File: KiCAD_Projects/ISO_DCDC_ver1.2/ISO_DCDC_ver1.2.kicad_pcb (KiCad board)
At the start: 2 copper layers, 60 x 60 mm, 51 parts, among them IC4 PC817, IC5 PC817, P1 CONN_01X01, P10 CONN_01X02, P12 CONN_01X01, P13 CONN_01X04, P14 CONN_01X02, P2 CONN_01X01, P21 CONN_01X02, P22 CONN_01X01, P23 CONN_01X01, P25 CONN_01X01, P26 CONN_01X01, P3 CONN_01X01, P4 CONN_01X02, P5 CONN_01X02, P6 CONN_01X02, P7 CONN_01X02, P8 CONN_01X01, Q1 MOSFET_N, U1 V23076-D3001-D142, U3 V23076-D3001-D142

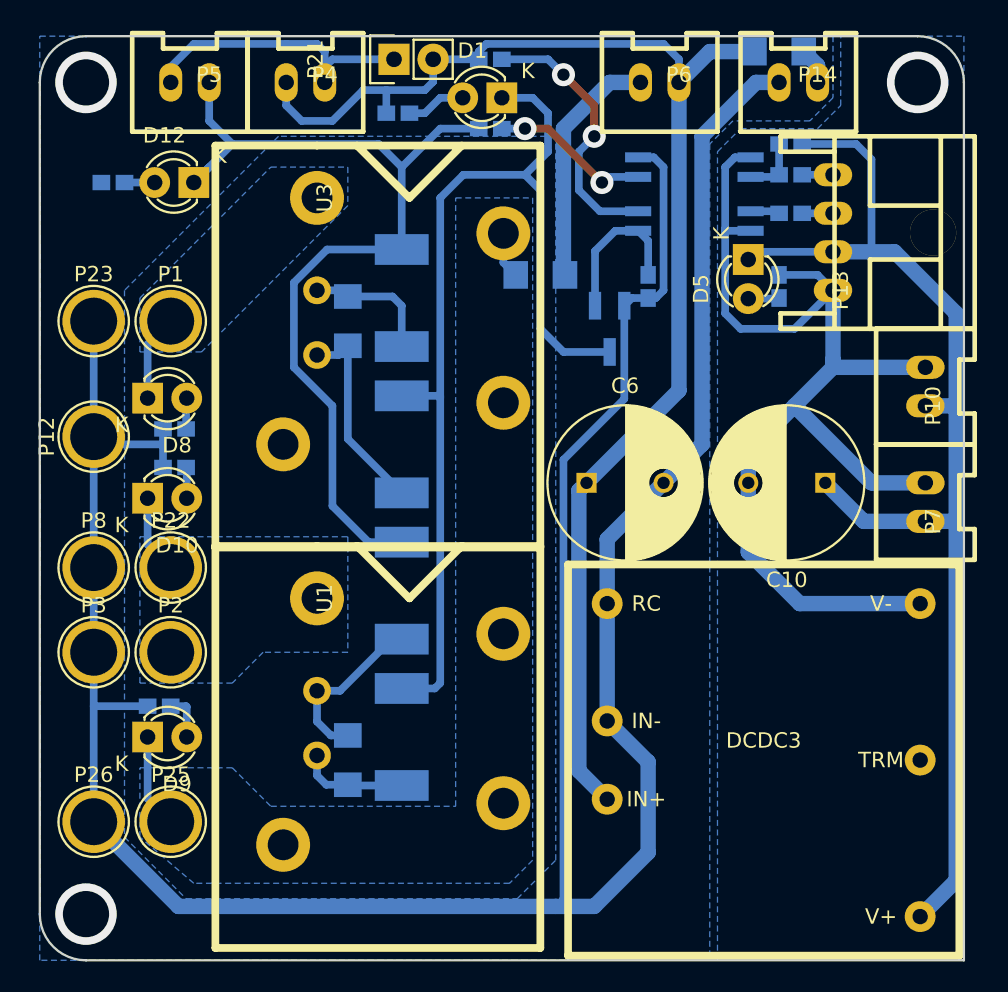
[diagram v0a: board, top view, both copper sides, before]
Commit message: 電源基板ver1.2加工した｡次ver1.3作るべきかも
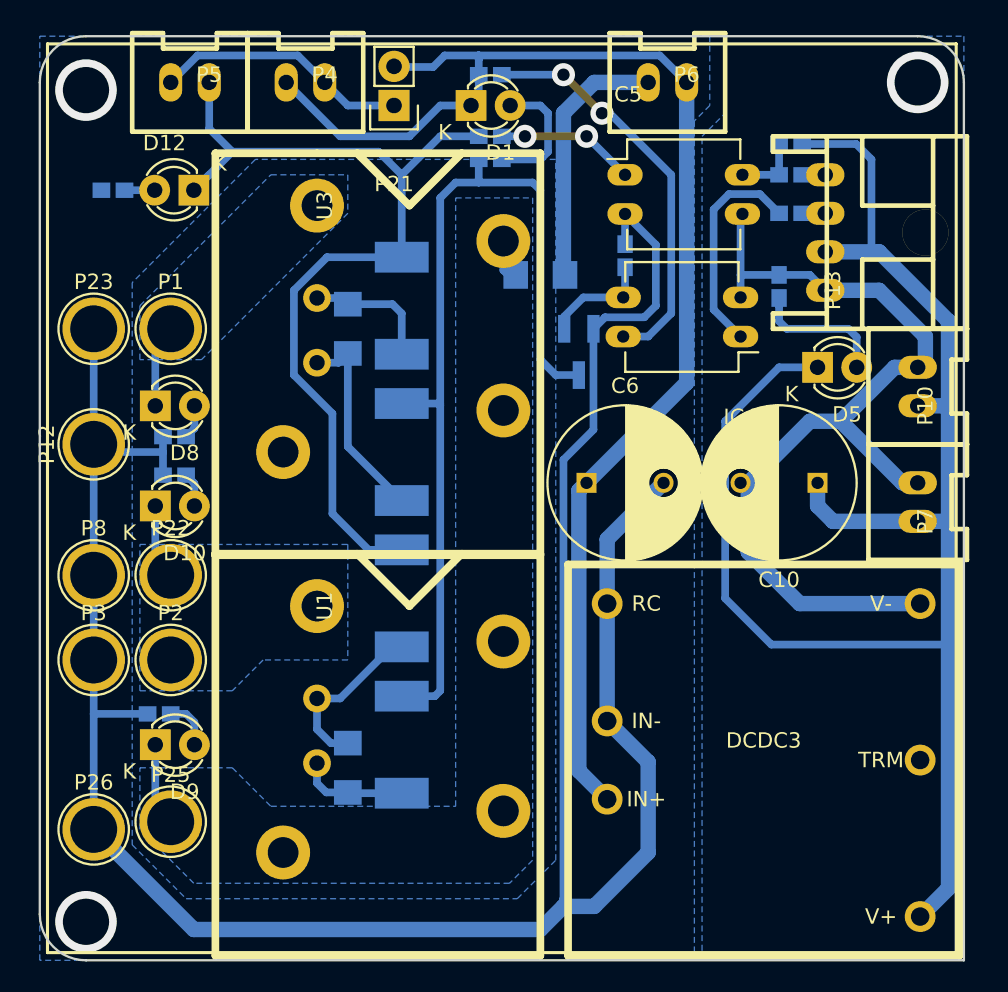
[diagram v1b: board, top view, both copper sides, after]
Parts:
- removed D4: DIODE, RP_KiCAD_Libs:C3216
- removed P14: CONN_01X02, RP_KiCAD_Connector:XA_2T
- IC4, IC5: footprint Housings_SOIC:SOIJ-4_5.3x5.3mm_Pitch1.27mm -> Housings_DIP:DIP-4_W7.62mm_LongPads_Slim; moved to F.Cu
- moved D5 8.32 mm to (50.5, 21.5), turned to 0 degrees
- moved IC4 8.08 mm to (45.5, 19.5)
- moved R1 6.71 mm to (29.0, 8.00)
- moved IC5 4.53 mm to (38.0, 9.00)
- moved P21 3.00 mm to (23.0, 4.50), turned to 180 degrees
- moved R11 2.92 mm to (38.0, 14.0), turned to 90 degrees
- moved Q1 2.50 mm to (35.0, 20.5)
- moved D1 2.06 mm to (28.0, 4.50), turned to 0 degrees
- moved R19 1.00 mm to (29.0, 2.50)
- moved D10 0.71 mm to (7.50, 30.5)
- moved D8 0.71 mm to (7.50, 24.0)
- moved D9 0.71 mm to (7.50, 46.0)
- moved C10 0.50 mm to (50.5, 29.0)
- moved D12 0.50 mm to (10.0, 10.0)
- moved D2 0.50 mm to (20.0, 47.5)
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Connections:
- D1 pad 1: /POWER_EN_LOW -> /15V
- R1 pad 2: /15V -> /POWER_EN_LOW
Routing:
- net GNDPWR: track 194.1 -> 163.3 mm
- net /12V: track 77.9 -> 107.3 mm
- net GND: track 75.0 -> 59.4 mm
- net Net-(IC4-Pad1): track 1.91 -> 14.3 mm
- net Net-(IC4-Pad4): track 17.6 -> 26.4 mm
- net Net-(D5-Pad2): track 2.02 -> 9.49 mm
- net /POWER_EN_LOW: track 66.5 -> 59.8 mm
- net Net-(D1-Pad2): track 3.87 -> 8.37 mm
- net Net-(IC4-Pad3): track 10.0 -> 7.15 mm
- net Net-(D4-Pad2): track 2.37 -> 0.00 mm
- net /15V: track 89.8 -> 88.0 mm
- net Net-(IC5-Pad1): track 10.5 -> 9.04 mm
- net Net-(D3-Pad1): track 15.8 -> 16.9 mm
- net Net-(P21-Pad1): track 19.5 -> 18.6 mm
- net +BATT: track 9.95 -> 9.25 mm
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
